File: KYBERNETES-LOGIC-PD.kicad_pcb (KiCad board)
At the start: 4 copper layers, 59.9 x 35.7 mm, 33 parts, among them J1 Logic Battery, J10 Battery Low, J2 Regulator In, J3 Regulator Out, J4 Regulator Enable, J5 I2C, J6 USB_C_Receptacle_PowerOnly_6P, J7 USB_C_Receptacle_PowerOnly_6P, J8 USB_C_Receptacle_PowerOnly_6P, J9 USB_C_Receptacle_PowerOnly_6P, U1 LM4040CEM3-3.0T, U2 LM2903, U3 INA219BxD, U4 LP2985-3.3

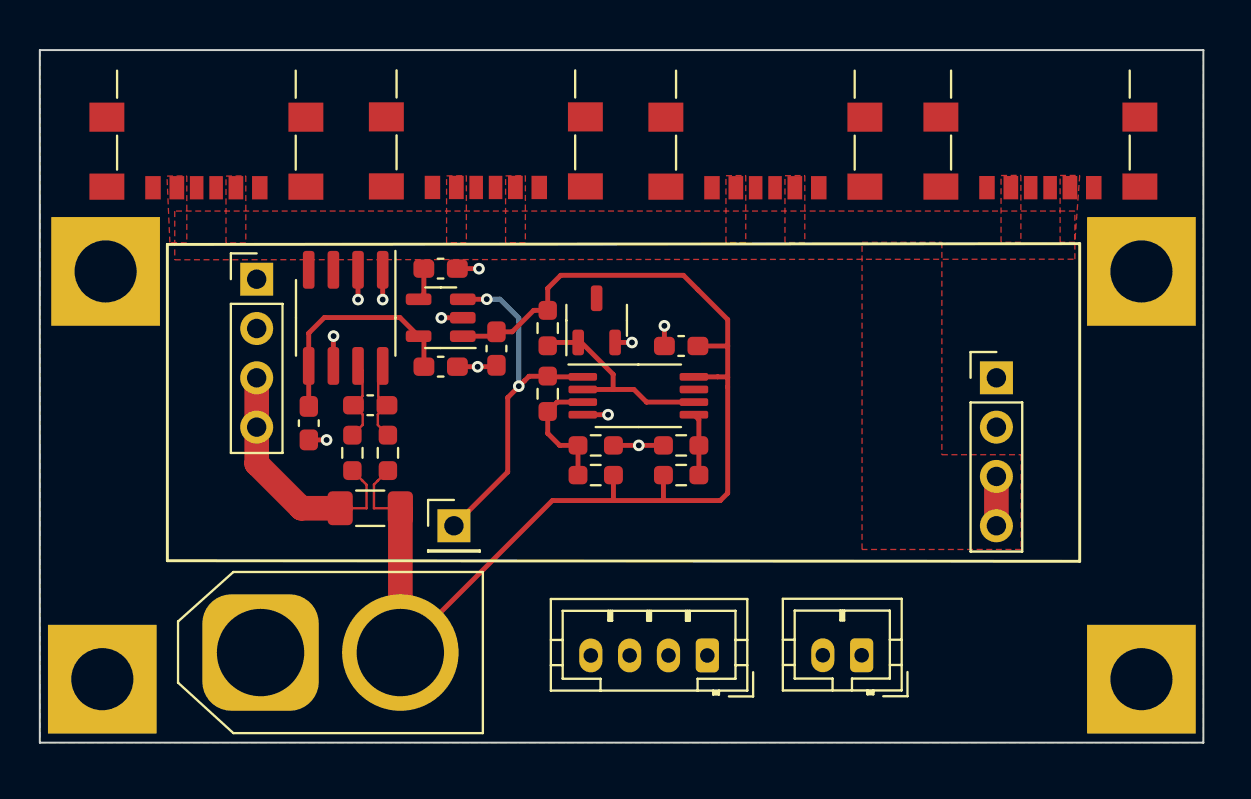
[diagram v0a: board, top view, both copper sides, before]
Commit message: more work
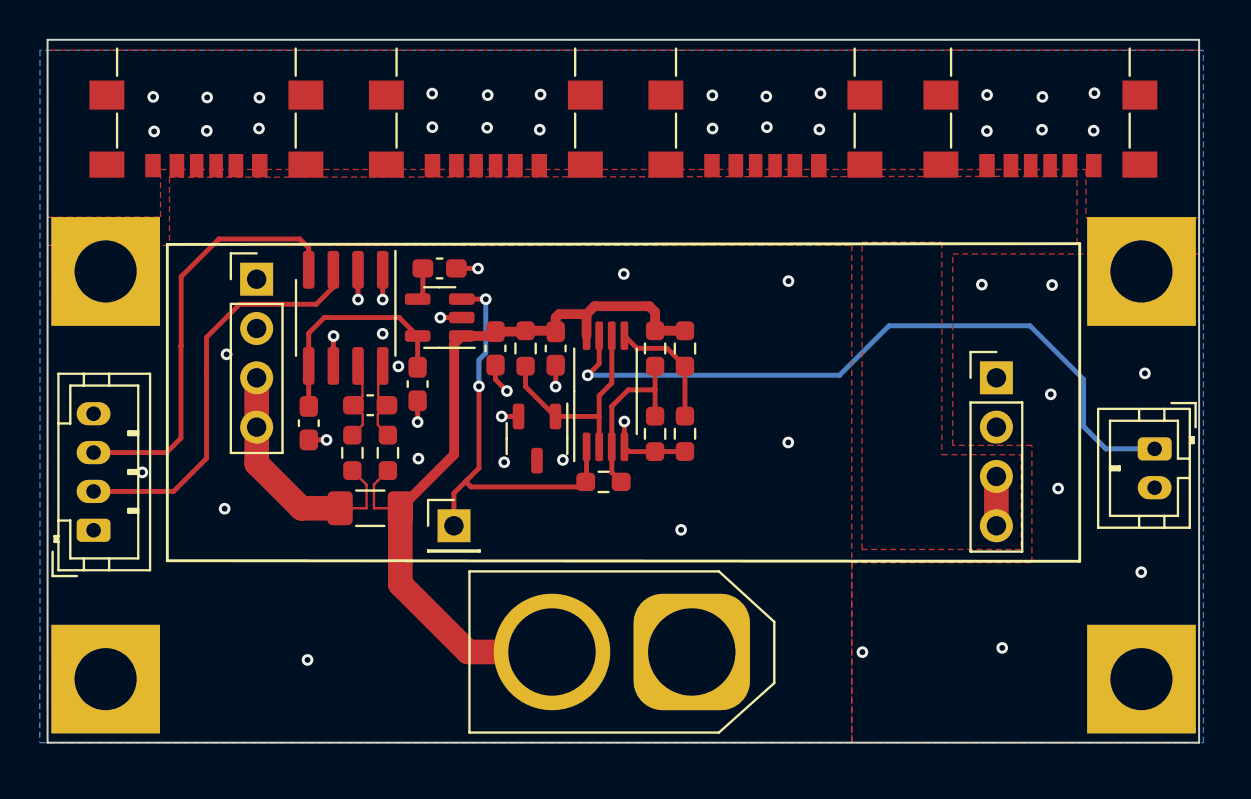
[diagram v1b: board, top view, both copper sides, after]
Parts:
- moved J5 32.3 mm to (118.2, 89.3), turned to 90 degrees
- moved J1 22.2 mm to (149.0, 95.6), turned to 180 degrees
- moved J10 18.5 mm to (172.9, 85.1), turned to -90 degrees
- moved R3 7.20 mm to (147.1, 79.9), turned to -90 degrees
- moved U1 6.82 mm to (141.0, 84.6), turned to -90 degrees
- moved R1 6.52 mm to (148.7, 80.0), turned to -90 degrees
- moved C1 6.46 mm to (142.0, 79.9), turned to -90 degrees
- moved R5 5.37 mm to (144.5, 86.8), turned to 180 degrees
- moved R4 3.11 mm to (147.1, 84.3), turned to -90 degrees
- moved U2 1.71 mm to (144.6, 82.2), turned to 90 degrees
- moved R6 1.55 mm to (140.5, 79.9)
- moved C3 1.49 mm to (134.9, 81.8), turned to -90 degrees
- moved J6 1.14 mm to (124.0, 67.5)
- moved J8 1.14 mm to (152.8, 67.5)
- moved J9 1.13 mm to (167.0, 67.5)
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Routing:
- net Net-(J10-Pin_1): track 0.00 -> 36.6 mm, vias 0 -> 1
- net SCL: track 0.00 -> 21.8 mm
- net SDA: track 0.00 -> 21.3 mm
- net +12V: track 63.0 -> 42.0 mm
- net LogicBattLowSense: track 3.22 -> 6.34 mm
- net REGULATOR_EN: track 18.9 -> 21.8 mm
- net LogicBattCritSense: track 6.48 -> 9.25 mm
- net GND: track 15.6 -> 17.0 mm, vias 11 -> 56
- net LogicBattRef: track 10.9 -> 11.6 mm
- added copper zone on F.Cu, net GND
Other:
- board size 59.9 x 35.7 mm -> 59.3 x 36.2 mm

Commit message: derp
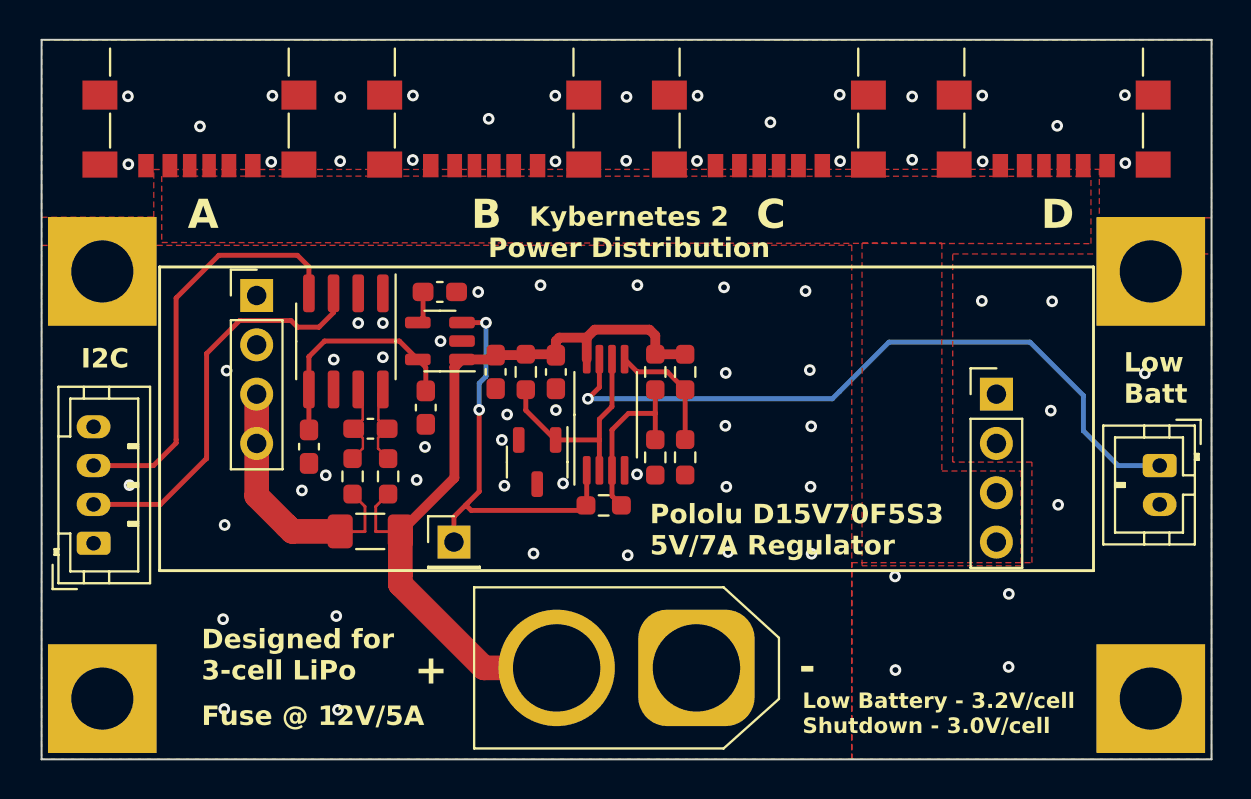
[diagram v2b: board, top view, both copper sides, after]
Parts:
- H1, H2, H3, H4: footprint MountingHole:MountingHole_3.2mm_M3_DIN965_Pad -> Footprints:MountingHole_3.2mm_M3_Pad_Square
- moved C3 1.28 mm to (135.3, 83.0)
- moved C6 1.21 mm to (138.9, 81.2)
- moved R4 1.21 mm to (147.1, 85.6)
- moved R5 1.21 mm to (144.5, 88.0)
- moved C1 1.21 mm to (142.0, 81.2)
- moved C2 1.21 mm to (129.3, 85.0)
- moved R1 1.21 mm to (148.7, 81.2)
- moved R2 1.21 mm to (148.7, 85.6)
- moved R9 1.21 mm to (131.6, 86.5)
- moved U2 1.21 mm to (144.6, 83.4)
- moved U3 1.21 mm to (131.2, 79.6)
- moved U4 1.21 mm to (136.0, 79.6)
- moved C4 1.21 mm to (136.0, 77.0)
- moved C5 1.21 mm to (132.5, 84.1)
- moved R3 1.21 mm to (147.1, 81.2)
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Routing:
- net GND: track 17.0 -> 0.14 mm, vias 56 -> 72
- net +5V: track 2.54 -> 0.00 mm
- net +12V: track 42.0 -> 41.0 mm
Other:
- board size 59.3 x 36.2 mm -> 60.3 x 37.1 mm
- board text added: "+"
- board text added: "-"
- board text added: "A"
- board text added: "B"
- board text added: "C"
- board text added: "D"
- board text added: "Designed for 3-cell LiPo"
- board text added: "Fuse @ 12V/5A"
- board text added: "I2C"
- board text added: "Kybernetes 2 Power Distribution"
- board text added: "Low Batt"
- board text added: "Low Battery - 3.2V/cell Shutdown - 3.0V/cell"
- board text added: "Pololu D15V70F5S3 5V/7A Regulator"

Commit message: first version for manufacturing
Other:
- copper layers 4 -> 2
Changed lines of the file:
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@@
 (kicad_pcb (version 20221018) (generator pcbnew)
   (general
-    (thickness 1.62684)
+    (thickness 1.61)
   )
   (paper "A4")
   (layers
     (0 "F.Cu" signal)
-    (1 "In1.Cu" power)
-    (2 "In2.Cu" power)
     (31 "B.Cu" signal)
     (32 "B.Adhes" user "B.Adhesive")
@@
       (layer "F.SilkS" (type "Top Silk Screen"))
       (layer "F.Paste" (type "Top Solder Paste"))
-      (layer "F.Mask" (type "Top Solder Mask") (thickness 0.02032))
+      (layer "F.Mask" (type "Top Solder Mask") (thickness 0.02))
       (layer "F.Cu" (type "copper") (thickness 0.035))
-      (layer "dielectric 1" (type "prepreg") (thickness 0.2104) (material "FR4") (epsilon_r 4.6) (loss_tangent 0.02))
-      (layer "In1.Cu" (type "copper") (thickness 0.0152))
-      (layer "dielectric 2" (type "core") (thickness 1.065) (material "FR4") (epsilon_r 4.6) (loss_tangent 0.02))
-      (layer "In2.Cu" (type "copper") (thickness 0.0152))
-      (layer "dielectric 3" (type "prepreg") (thickness 0.2104) (material "FR4") (epsilon_r 4.6) (loss_tangent 0.02))
+      (layer "dielectric 1" (type "core") (thickness 1.5) (material "FR4") (epsilon_r 4.5) (loss_tangent 0.02))
       (layer "B.Cu" (type "copper") (thickness 0.035))
-      (layer "B.Mask" (type "Bottom Solder Mask") (thickness 0.02032))
+      (layer "B.Mask" (type "Bottom Solder Mask") (thickness 0.02))
       (layer "B.Paste" (type "Bottom Solder Paste"))
       (layer "B.SilkS" (type "Bottom Silk Screen"))

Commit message: source needs 10 Kohm pullups to advertise 3A capability
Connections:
- J6 pad A5: unconnected-(J6-CC1-PadA5) -> Net-(J6-CC1)
- J6 pad B5: unconnected-(J6-CC2-PadB5) -> Net-(J6-CC2)
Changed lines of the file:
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@@
   (net 13 "SDA")
   (net 14 "SCL")
-  (net 15 "unconnected-(J6-CC1-PadA5)")
-  (net 16 "unconnected-(J6-CC2-PadB5)")
+  (net 15 "Net-(J6-CC1)")
+  (net 16 "Net-(J6-CC2)")
   (net 17 "unconnected-(J7-CC1-PadA5)")
   (net 18 "unconnected-(J7-CC2-PadB5)")
@@
       (stroke (width 0.1) (type solid)) (fill none) (layer "F.Fab"))
     (pad "A5" smd rect (at -0.5 -3.0325 180) (size 0.7 1.2) (layers "F.Cu" "F.Paste" "F.Mask")
-      (net 15 "unconnected-(J6-CC1-PadA5)") (pinfunction "CC1") (pintype "bidirectional+no_connect"))
+      (net 15 "Net-(J6-CC1)") (pinfunction "CC1") (pintype "bidirectional"))
     (pad "A9" smd rect (at 1.52 -3.0325) (size 0.76 1.2) (layers "F.Cu" "F.Paste" "F.Mask")
       (net 3 "+5V") (pinfunction "VBUS") (pintype "passive"))
@@
       (net 1 "GND") (pinfunction "GND") (pintype "passive"))
     (pad "B5" smd rect (at 0.5 -3.0325) (size 0.7 1.2) (layers "F.Cu" "F.Paste" "F.Mask")
-      (net 16 "unconnected-(J6-CC2-PadB5)") (pinfunction "CC2") (pintype "bidirectional+no_connect"))
+      (net 16 "Net-(J6-CC2)") (pinfunction "CC2") (pintype "bidirectional"))
     (pad "B9" smd rect (at -1.52 -3.0325 180) (size 0.76 1.2) (layers "F.Cu" "F.Paste" "F.Mask")
       (net 3 "+5V") (pinfunction "VBUS") (pintype "passive"))
